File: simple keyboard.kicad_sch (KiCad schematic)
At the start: 18 parts, among them J1 USB_C_Receptacle_USB2.0_14P, SW1 SW_Push, SW2 SW_Push, SW3 SW_Push, U1 ATtiny25-20P

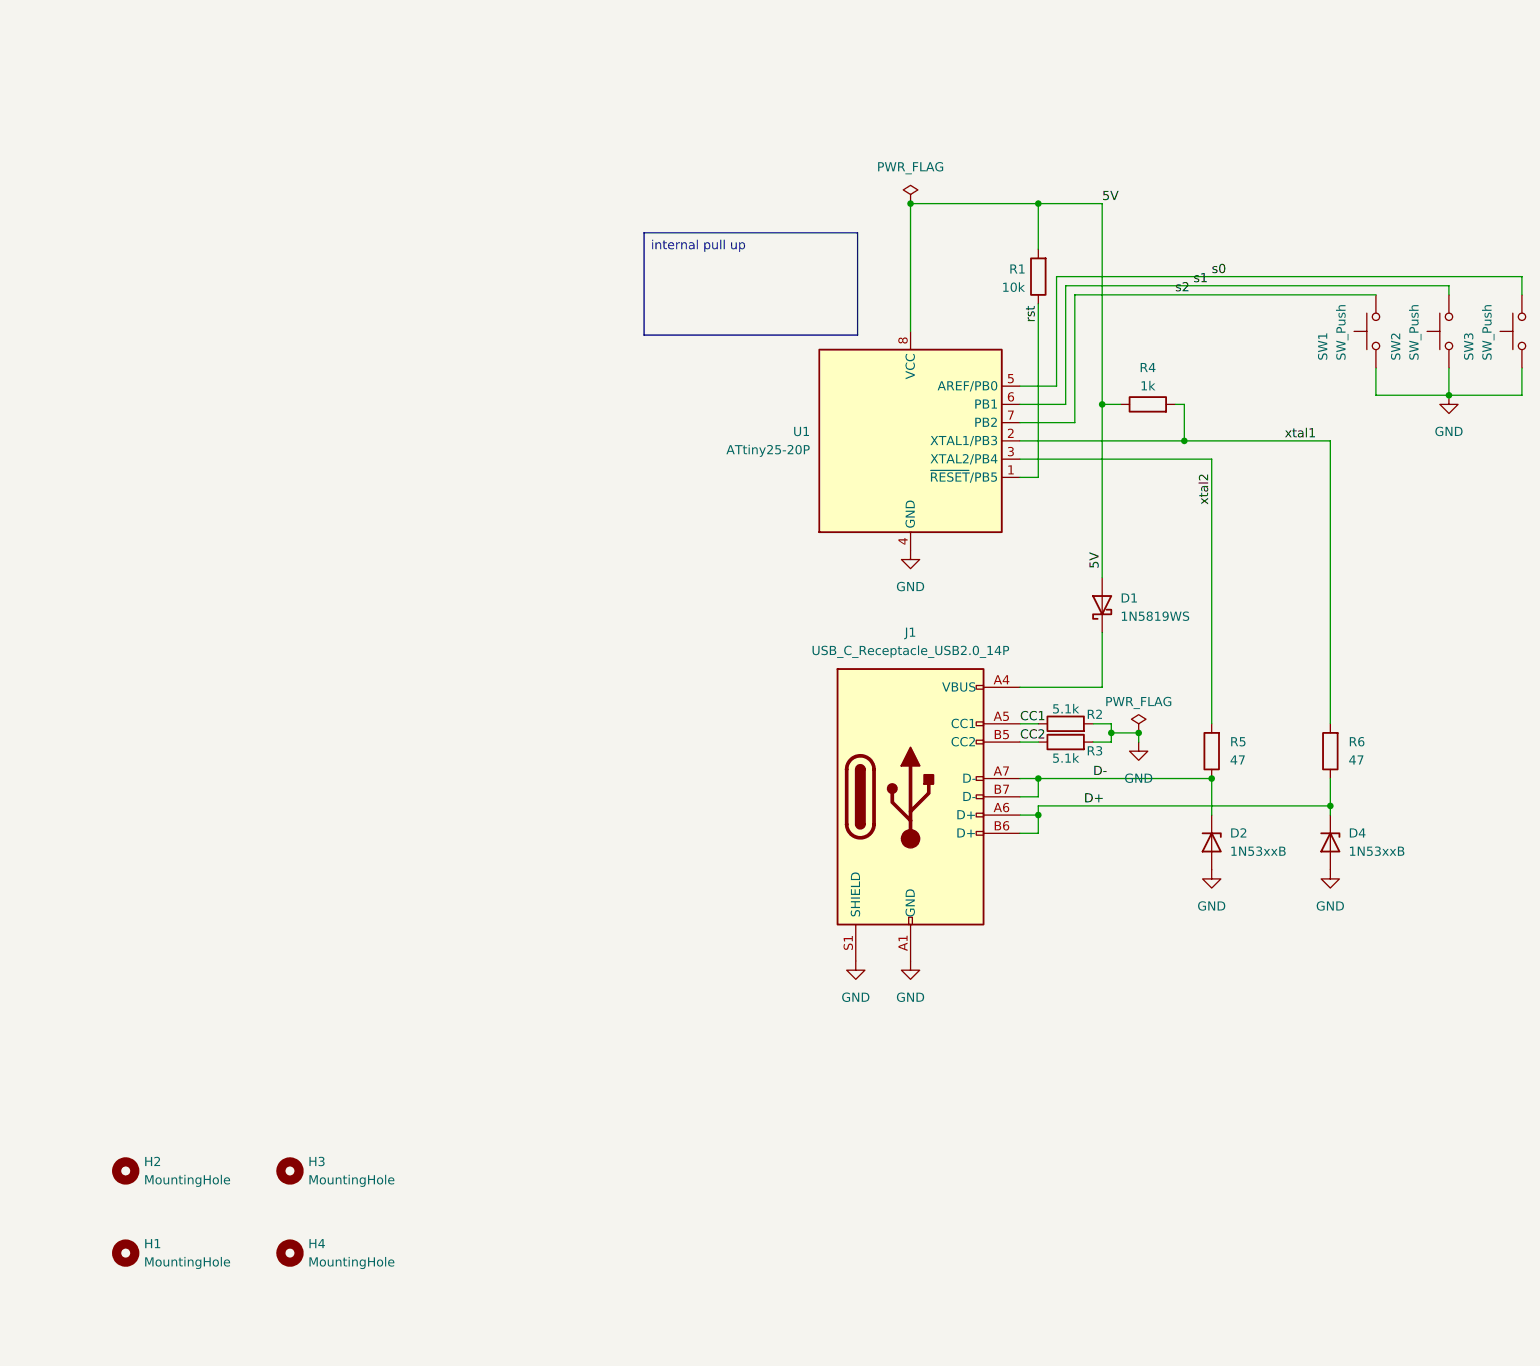
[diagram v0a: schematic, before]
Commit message: updata 29 3 26
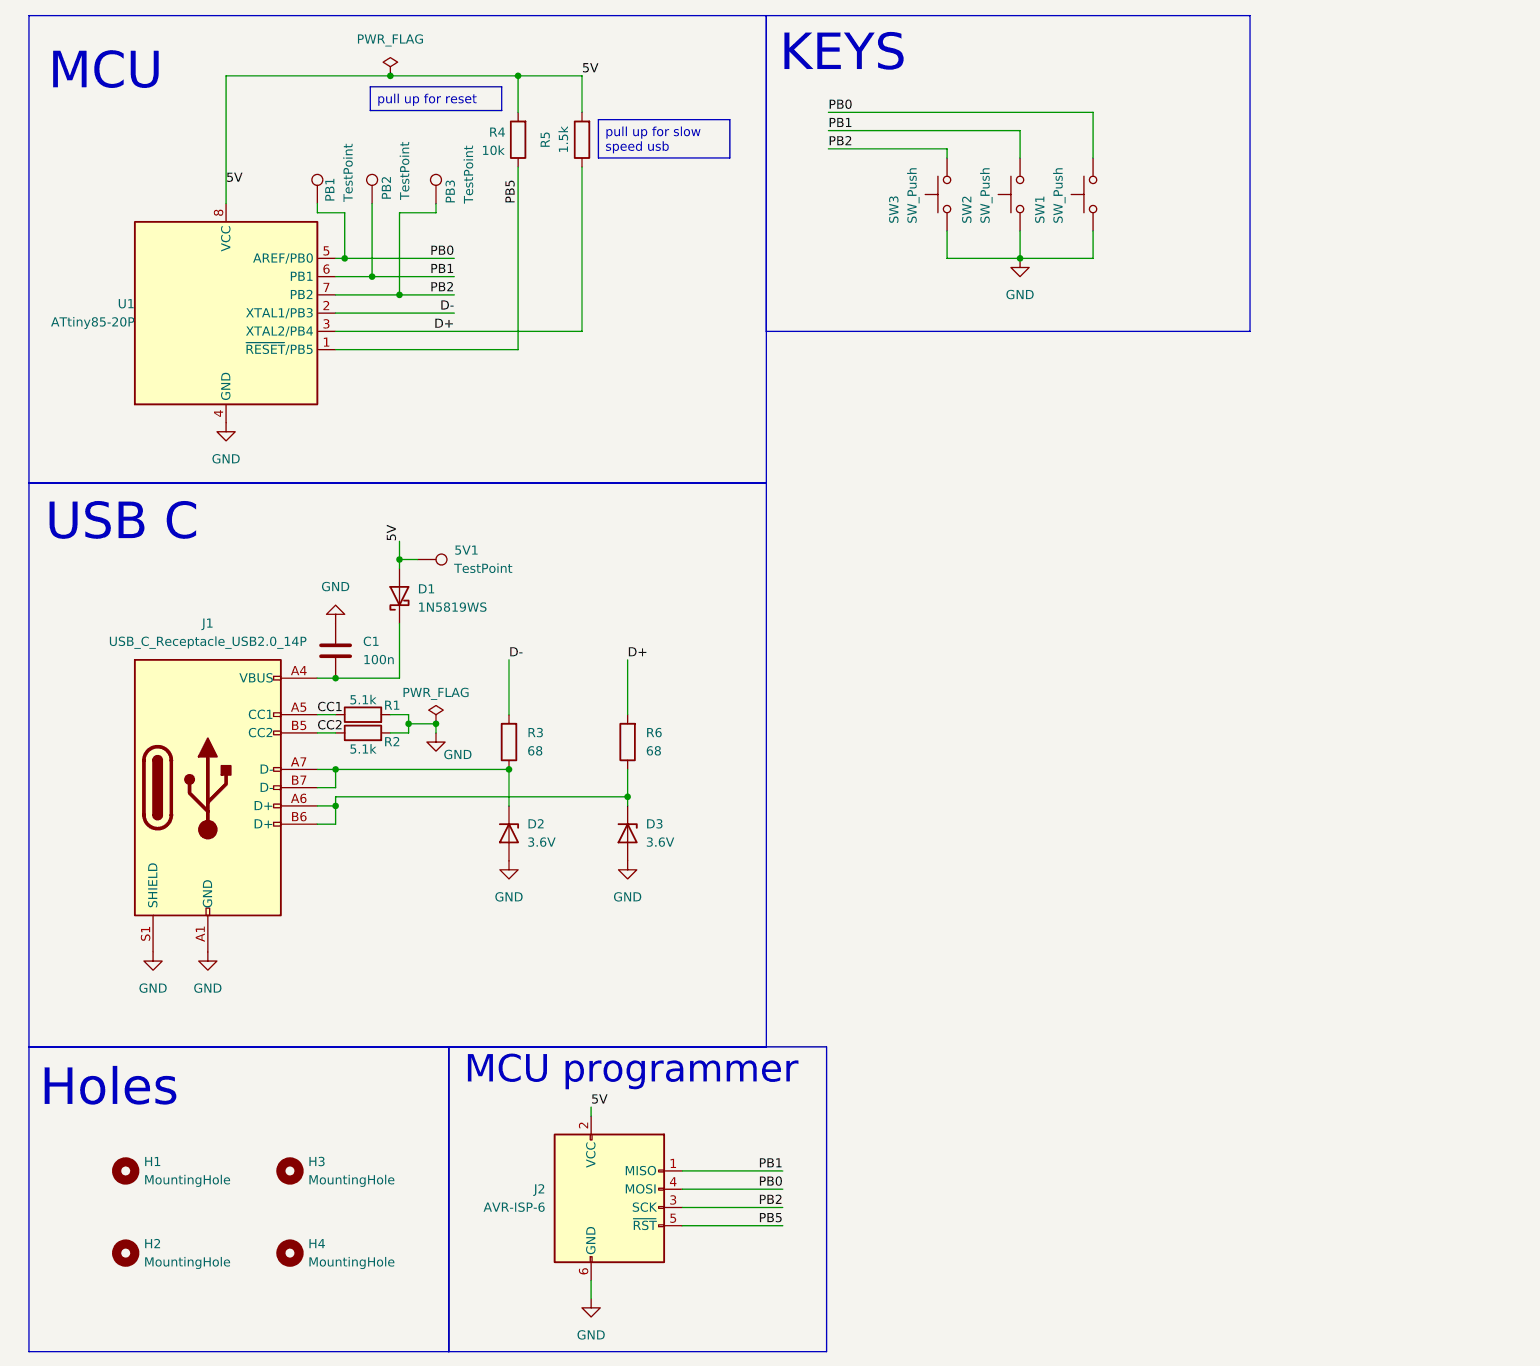
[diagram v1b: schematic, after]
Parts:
- removed U1: ATtiny25-20P, Package_DIP:DIP-8_W7.62mm, symbol MCU_Microchip_ATtiny:ATtiny25-20P
- added 5V1: TestPoint, TestPoint:TestPoint_Pad_1.0x1.0mm, symbol Connector:TestPoint
- added C1: 100n, Capacitor_Tantalum_SMD:CP_EIA-6032-28_Kemet-C, symbol Device:C
- added J2: AVR-ISP-6, 665306124022:665306124022, symbol Connector:AVR-ISP-6
- added PB1, PB2, PB3: TestPoint, TestPoint:TestPoint_Pad_D1.0mm, symbol Connector:TestPoint
- added U1: ATtiny85-20P, Package_DIP:DIP-8_W7.62mm, symbol MCU_Microchip_ATtiny:ATtiny85-20P
- D1: Part_num (none) -> 1N5819WS
- D2: value 1N53xxB -> 3.6V; footprint Diode_THT:D_DO-201_P15.24mm_Horizontal -> Diode_THT:D_DO-35_SOD27_P7.62mm_Horizontal; Part_num (none) -> TZX3V6C-TR
- D3: renamed from D4; value 1N53xxB -> 3.6V; footprint Diode_THT:D_DO-201_P15.24mm_Horizontal -> Diode_THT:D_DO-35_SOD27_P7.62mm_Horizontal; Part_num (none) -> TZX3V6C-TR
- R3: renamed from R5; value 47 -> 68; footprint Resistor_THT:R_Axial_DIN0207_L6.3mm_D2.5mm_P7.62mm_Horizontal -> Resistor_THT:R_Axial_DIN0204_L3.6mm_D1.6mm_P5.08mm_Horizontal; Part_num CFR-25JT-52-47R -> MFR25SFTF52-68R
- R5: renamed from R4; value 1k -> 1.5k
- R6: value 47 -> 68; footprint Resistor_THT:R_Axial_DIN0207_L6.3mm_D2.5mm_P7.62mm_Horizontal -> Resistor_THT:R_Axial_DIN0204_L3.6mm_D1.6mm_P5.08mm_Horizontal; Part_num CFR-25JT-52-47R -> MFR25SFTF52-68R
- renumbered H2 to H1, H1 to H2, R2 to R1, R3 to R2, R1 to R4, SW3 to SW1, SW1 to SW3
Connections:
- net xtal2 is gone; now on net D-: R3.2
- net 5V: now also R5.2, 5V1.1, J2.2 (VCC), U1.8 (VCC); no longer R5.1
- net D+: now also R5.1, R6.2, U1.3 (XTAL2/PB4); no longer D3.1 (K), J1.A6 (D+), J1.B6 (D+), R6.1
- net D-: now also U1.2 (XTAL1/PB3); no longer D2.1 (K), J1.A7 (D-), J1.B7 (D-), R3.1
- net GND: now also C1.1, J2.6 (GND), U1.4 (GND)
- net at D1.1 (K), J1.A4 (VBUS), J1.A9 (VBUS)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: now also C1.2
- net rst renamed PB5
- net PB5: now also J2.5 (~{RST}), U1.1 (~{RESET}/PB5)
- net s0 renamed PB0
- net PB0: now also J2.4 (MOSI), PB1.1, U1.5 (AREF/PB0)
- net s1 renamed PB1
- net PB1: now also J2.1 (MISO), PB2.1, U1.6 (PB1)
- net s2 renamed PB2
- net PB2: now also J2.3 (SCK), PB3.1, U1.7 (PB2)
- removed net xtal1: R5.2, R6.2
- new net: D2.1 (K), J1.A7 (D-), J1.B7 (D-), R3.1
- new net: D3.1 (K), J1.A6 (D+), J1.B6 (D+), R6.1
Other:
- note added: "Holes"
- note added: "KEYS"
- note added: "MCU"
- note added: "MCU programmer"
- note added: "USB C"
- moved on the sheet: D1, D2, D3, J1, R1, R2, R3, R4, R5, R6, SW1, SW2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
